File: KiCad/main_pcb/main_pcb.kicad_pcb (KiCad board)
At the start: 2 copper layers, 130 x 100 mm, 61 parts, among them J1 Conn_01x07, J2 Conn_01x07, J3 Conn_01x13, J4 Conn_01x06, J5 Conn_01x02, J6 USB_C_Receptacle_USB2.0_14P, SW1 SW_Push, U1 TXB0104D, U2 TXB0104D, U3 TXB0104D, U4 ATmega2560-16A, U5 AMS1117-3.3, U7 CH340C, Y1 Crystal_GND24

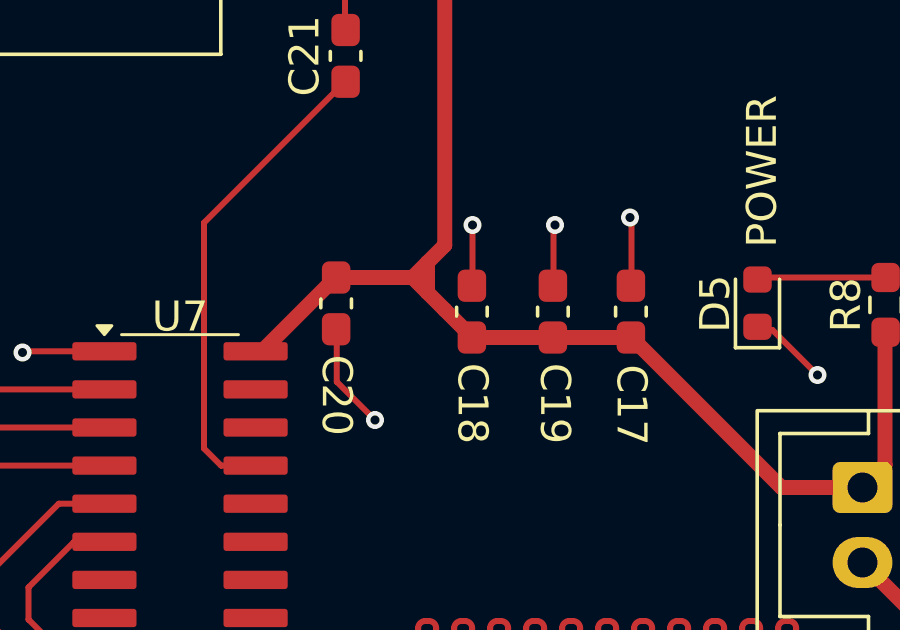
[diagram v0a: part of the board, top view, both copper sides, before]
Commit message: feat(pcb): Should be a-ok
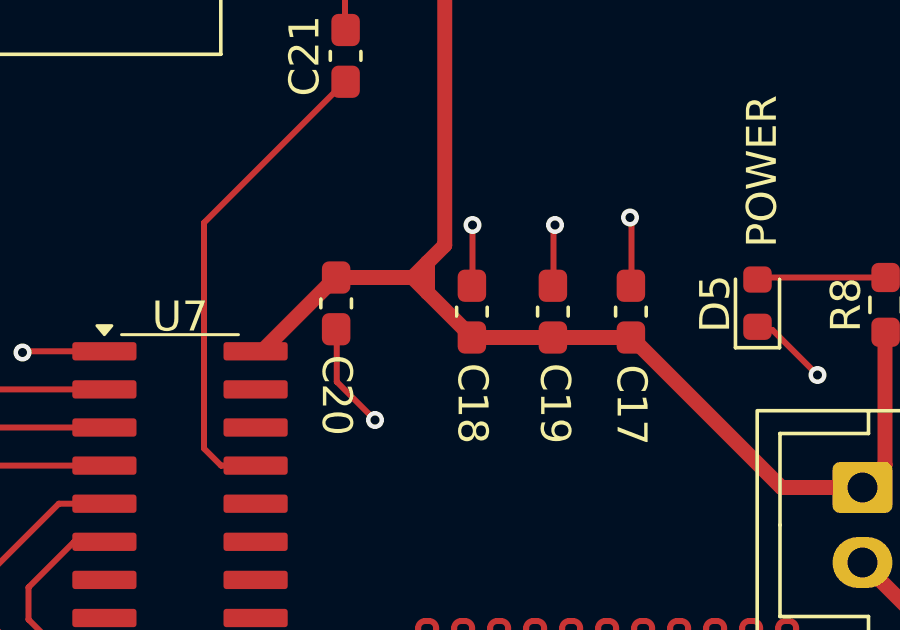
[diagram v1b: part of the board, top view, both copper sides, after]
